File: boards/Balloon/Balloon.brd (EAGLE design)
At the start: 41.9 x 69.8 mm, 23 parts

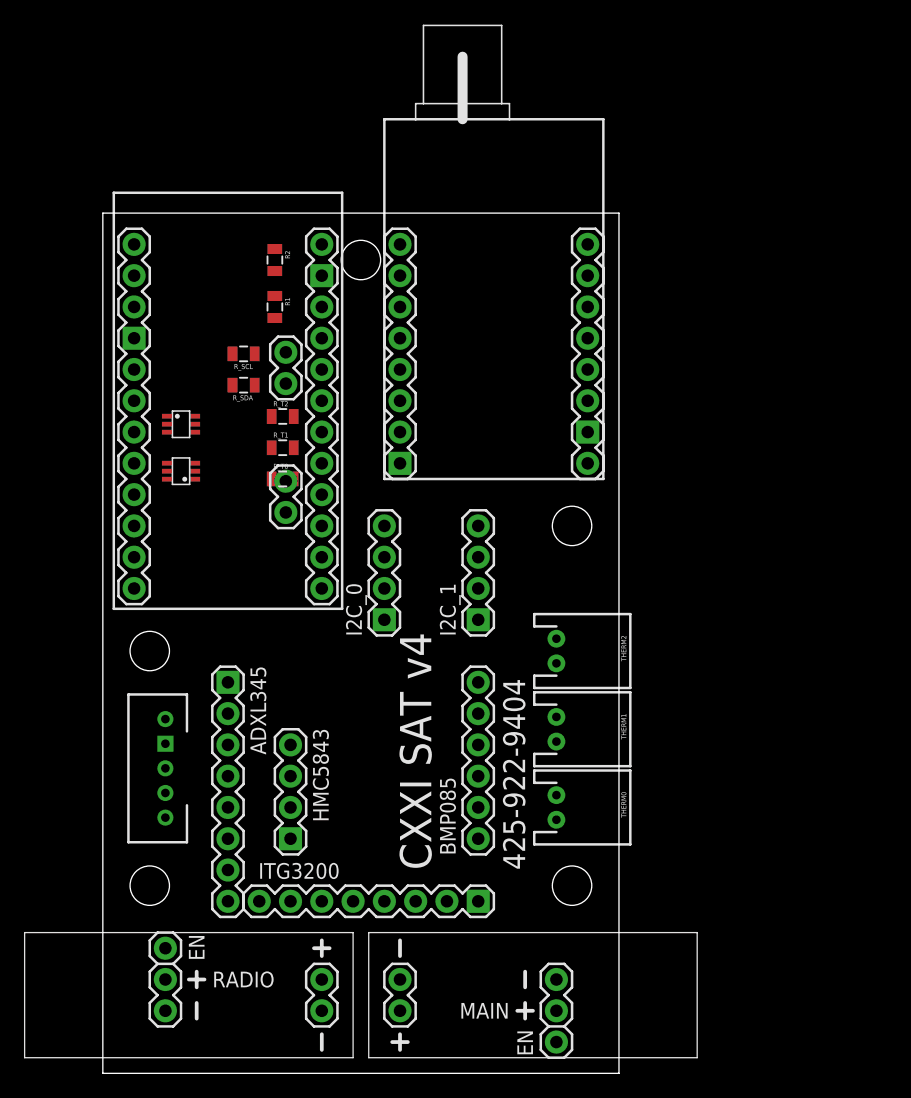
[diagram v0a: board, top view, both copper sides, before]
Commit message: Ballon v4 as submitted to manufacturing
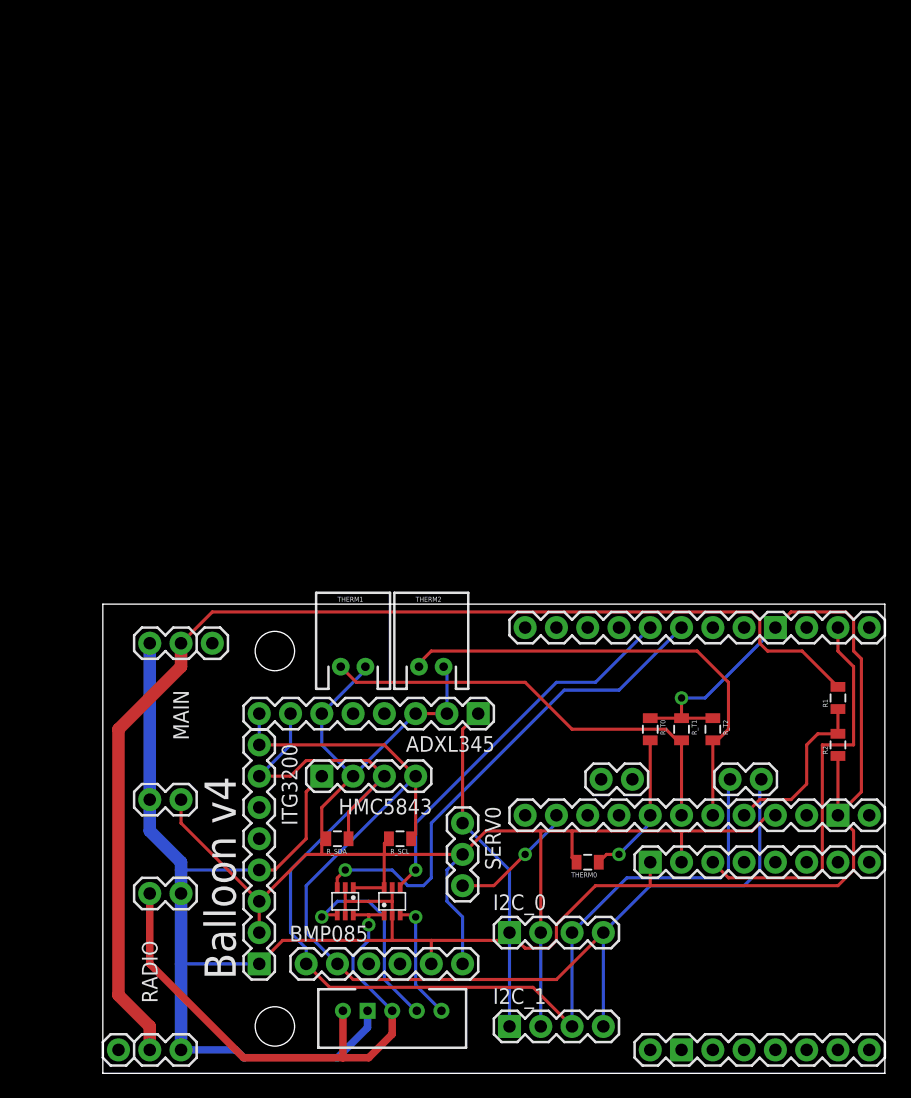
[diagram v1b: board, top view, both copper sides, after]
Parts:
- added SERV0: (no value), SparkFun-Connectors:1X03
- ARDUINO: value ARDUINO_PRO_MINI -> ARDUINO_PRO_MINI-NOSILK; device OpenSpace:ARDUINO_PRO_MINI -> OpenSpace:ARDUINO_PRO_MINI-NOSILK
- GPS: value VENUS_GPS -> VENUS_GPS-NOSILK; device OpenSpace:VENUS_GPS -> OpenSpace:VENUS_GPS-NOSILK
- MAIN, RADIO: device OpenSpace:POWER-TPS6300X -> OpenSpace:POWER-TPS6300X-NOSILK
- R1: value (none) -> 1.2K
- R2: value (none) -> 3.9K
- THERM0: device SparkFun-Connectors:JST-2-PTH -> SparkFun-Passives:0805
- moved R2 60.3 mm to (59.7, 26.7), turned to 90 degrees
- moved R1 55.7 mm to (59.7, 30.5), turned to 90 degrees
- moved GPS 53.4 mm to (53.3, 9.53), turned to 270 degrees
- moved ARDUINO 45.4 mm to (48.3, 28.6), turned to 270 degrees
- moved R_T2 43.2 mm to (49.5, 27.9), turned to 270 degrees
- moved R_SCL 41.4 mm to (24.1, 19.1)
- moved SHIFT_FROM_RADIO 41.0 mm to (19.7, 14.0), turned to 180 degrees
- moved R_T1 39.6 mm to (47.0, 27.9), turned to 270 degrees
- moved MAIN 39.1 mm to (5.08, 32.4), turned to 270 degrees
- moved SHIFT_TO_RADIO 38.9 mm to (23.5, 14.0), turned to 0 degrees
- moved R_SDA 37.6 mm to (19.1, 19.1)
- moved R_T0 36.1 mm to (44.5, 27.9), turned to 270 degrees
- moved I2C_1 33.1 mm to (33.0, 3.81), turned to 0 degrees
- moved I2C_0 27.4 mm to (33.0, 11.4), turned to 0 degrees
- moved XTEND 27.0 mm to (23.5, 5.08), turned to 180 degrees
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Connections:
- new net D11: ARDUINO.D11*, SERV0.3
- net 3.3V: now also SERV0.2
- net GND: now also SERV0.1
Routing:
- net GND: track 0.00 -> 220.4 mm, vias 0 -> 1
- net 3.3V: track 0.00 -> 128.9 mm
- net SDA: track 0.00 -> 96.1 mm
- net SCL: track 0.00 -> 95.0 mm
- net 1.8V: track 0.00 -> 94.2 mm
- net 5V: track 0.00 -> 47.2 mm, vias 0 -> 1
- net D4: track 0.00 -> 40.8 mm, vias 0 -> 1
- net A2: track 0.00 -> 38.4 mm
- net A1: track 0.00 -> 36.2 mm
- net RX: track 0.00 -> 32.4 mm
- net D5: track 0.00 -> 31.4 mm, vias 0 -> 1
- net N$1: track 0.00 -> 16.2 mm, vias 0 -> 1
- net N$2: track 0.00 -> 14.2 mm
- net A0: track 0.00 -> 12.2 mm, vias 0 -> 1
- net D11: track 0.00 -> 10.4 mm, vias 0 -> 1
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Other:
- board size 41.9 x 69.8 mm -> 63.5 x 38.1 mm
- board text added: "Balloon v4"
- board text removed: "425-922-9404"
- board text removed: "CXXI SAT v4"
